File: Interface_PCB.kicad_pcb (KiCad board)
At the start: 2 copper layers, 46.5 x 47.9 mm, 46 parts, among them IC1 STM32L412RBT6P, U1 AMS1117-3.3, Y1 Crystal, Y2 Crystal

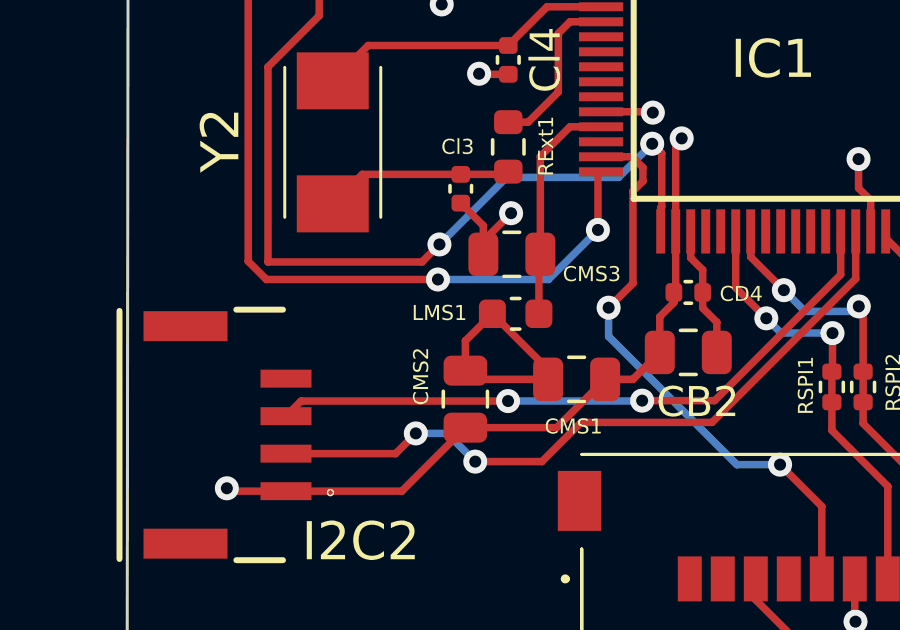
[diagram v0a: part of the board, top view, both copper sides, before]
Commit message: Added BOM, position and gerber files
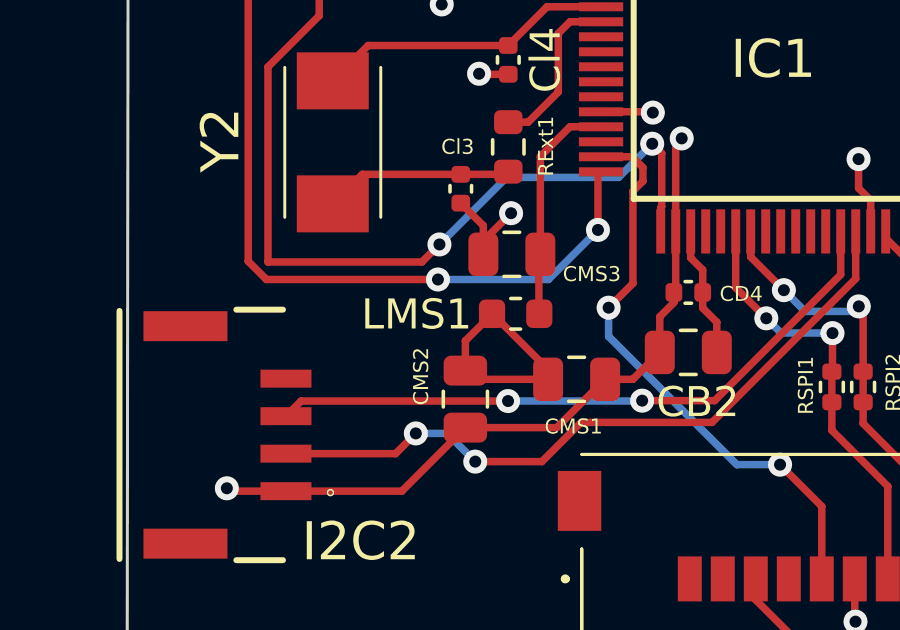
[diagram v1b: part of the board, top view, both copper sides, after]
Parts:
- LMS1: footprint Capacitor_SMD:C_0603_1608Metric -> Inductor_SMD:L_0603_1608Metric
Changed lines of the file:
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@@
       (drillshape 0)
       (scaleselection 1)
-      (outputdirectory "drill files/")
+      (outputdirectory "drill files/gerber/")
     )
   )
@@
     )
     (fp_line (start -4.65 -4.65) (end 4.65 -4.65) (layer "F.SilkS") (width 0.2))
-    (fp_line (start -4.65 4.65) (end -4.65 -4.65) (layer "F.SilkS") (width 0.2))
     (fp_line (start 4.65 4.65) (end -4.65 4.65) (layer "F.SilkS") (width 0.2))
+    (fp_line (start -4.65 4.65) (end -4.65 -4.65) (layer "F.SilkS") (width 0.2))
     (fp_line (start 4.65 -4.65) (end 4.65 4.65) (layer "F.SilkS") (width 0.2))
     (fp_circle (center -6.225 -4.5) (end -6.225 -4.375) (layer "F.SilkS") (width 0.25) (fill none))
-    (fp_line (start -6.725 -6.725) (end 6.725 -6.725) (layer "F.CrtYd") (width 0.05))
     (fp_line (start 6.725 -6.725) (end 6.725 6.725) (layer "F.CrtYd") (width 0.05))
-    (fp_line (start -6.725 6.725) (end -6.725 -6.725) (layer "F.CrtYd") (width 0.05))
     (fp_line (start 6.725 6.725) (end -6.725 6.725) (layer "F.CrtYd") (width 0.05))
+    (fp_line (start -6.725 -6.725) (end 6.725 -6.725) (layer "F.CrtYd") (width 0.05))
+    (fp_line (start -6.725 6.725) (end -6.725 -6.725) (layer "F.CrtYd") (width 0.05))
+    (fp_line (start -5 -4.5) (end -4.5 -5) (layer "F.Fab") (width 0.1))
+    (fp_line (start 5 -5) (end 5 5) (layer "F.Fab") (width 0.1))
     (fp_line (start -5 5) (end -5 -5) (layer "F.Fab") (width 0.1))
     (fp_line (start -5 -5) (end 5 -5) (layer "F.Fab") (width 0.1))
     (fp_line (start 5 5) (end -5 5) (layer "F.Fab") (width 0.1))
-    (fp_line (start 5 -5) (end 5 5) (layer "F.Fab") (width 0.1))
-    (fp_line (start -5 -4.5) (end -4.5 -5) (layer "F.Fab") (width 0.1))
     (pad "1" smd rect locked (at -5.738 -3.75 90) (size 0.3 1.475) (layers "F.Cu" "F.Paste" "F.Mask")
       (net 3 "+3V3") (pinfunction "VBAT") (pintype "passive"))
@@
     (pad "" np_thru_hole circle (at 0 0) (size 2.1 2.1) (drill 2.1) (layers *.Cu *.Mask))
   )
-  (footprint "Capacitor_SMD:C_0603_1608Metric" (layer "F.Cu")
+  (footprint "Inductor_SMD:L_0603_1608Metric" (layer "F.Cu")
     (at 127.0508 111.506)
-    (descr "Capacitor SMD 0603 (1608 Metric), square (rectangular) end terminal, IPC_7351 nominal, (Body size source: IPC-SM-782 page 76, https://www.pcb-3d.com/wordpress/wp-content/uploads/ipc-sm-782a_amendment_1_and_2.pdf), generated with kicad-footprint-generator")
-    (tags "capacitor")
+    (descr "Inductor SMD 0603 (1608 Metric), square (rectangular) end terminal, IPC_7351 nominal, (Body size source: http://www.tortai-tech.com/upload/download/2011102023233369053.pdf), generated with kicad-footprint-generator")
+    (tags "inductor")
     (property "Sheetfile" "Interface_PCB.kicad_sch")
     (property "Sheetname" "")
     (attr smd)
-    (fp_text reference "LMS1" (at -2.54 -0.0254 180) (layer "F.SilkS")
-      (effects (font (size 0.5 0.5) (thickness 0.125)))
+    (fp_text reference "LMS1" (at -3.302 0.0254) (layer "F.SilkS")
+      (effects (font (size 1 1) (thickness 0.15)))
     )
     (fp_text value "39nH" (at 0 1.43) (layer "F.Fab")
@@
       (effects (font (size 0.4 0.4) (thickness 0.06)))
     )
-    (fp_line (start -0.14058 -0.51) (end 0.14058 -0.51) (layer "F.SilkS") (width 0.12))
-    (fp_line (start -0.14058 0.51) (end 0.14058 0.51) (layer "F.SilkS") (width 0.12))
+    (fp_line (start -0.162779 -0.51) (end 0.162779 -0.51) (layer "F.SilkS") (width 0.12))
+    (fp_line (start -0.162779 0.51) (end 0.162779 0.51) (layer "F.SilkS") (width 0.12))
     (fp_line (start -1.48 -0.73) (end 1.48 -0.73) (layer "F.CrtYd") (width 0.05))
-    (fp_line (start 1.48 -0.73) (end 1.48 0.73) (layer "F.CrtYd") (width 0.05))
     (fp_line (start -1.48 0.73) (end -1.48 -0.73) (layer "F.CrtYd") (width 0.05))
+    (fp_line (start 1.48 -0.73) (end 1.48 0.73) (layer "F.CrtYd") (width 0.05))
     (fp_line (start 1.48 0.73) (end -1.48 0.73) (layer "F.CrtYd") (width 0.05))
-    (fp_line (start -0.8 0.4) (end -0.8 -0.4) (layer "F.Fab") (width 0.1))
+    (fp_line (start 0.8 -0.4) (end 0.8 0.4) (layer "F.Fab") (width 0.1))
     (fp_line (start -0.8 -0.4) (end 0.8 -0.4) (layer "F.Fab") (width 0.1))
+    (fp_line (start -0.8 0.4) (end -0.8 -0.4) (layer "F.Fab") (width 0.1))
     (fp_line (start 0.8 0.4) (end -0.8 0.4) (layer "F.Fab") (width 0.1))
-    (fp_line (start 0.8 -0.4) (end 0.8 0.4) (layer "F.Fab") (width 0.1))
-    (pad "1" smd roundrect (at -0.775 0) (size 0.9 0.95) (layers "F.Cu" "F.Paste" "F.Mask") (roundrect_rratio 0.25)
+    (pad "1" smd roundrect (at -0.7875 0) (size 0.875 0.95) (layers "F.Cu" "F.Paste" "F.Mask") (roundrect_rratio 0.25)
       (net 3 "+3V3") (pinfunction "1") (pintype "passive"))
-    (pad "2" smd roundrect (at 0.775 0) (size 0.9 0.95) (layers "F.Cu" "F.Paste" "F.Mask") (roundrect_rratio 0.25)
+    (pad "2" smd roundrect (at 0.7875 0) (size 0.875 0.95) (layers "F.Cu" "F.Paste" "F.Mask") (roundrect_rratio 0.25)
       (net 4 "+3.3VA") (pinfunction "2") (pintype "passive"))
-    (model "${KICAD6_3DMODEL_DIR}/Capacitor_SMD.3dshapes/C_0603_1608Metric.wrl"
+    (model "${KICAD6_3DMODEL_DIR}/Inductor_SMD.3dshapes/L_0603_1608Metric.wrl"
       (offset (xyz 0 0 0))
       (scale (xyz 1 1 1))
